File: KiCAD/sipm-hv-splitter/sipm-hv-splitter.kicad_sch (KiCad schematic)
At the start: 16 parts, among them J1 Conn_02x18_Odd_Even, J2 Conn_02x17_Odd_Even, J3 -OMIT-, U1 ATmega328-M, U14 TPS7A25, U16 TPS7A25

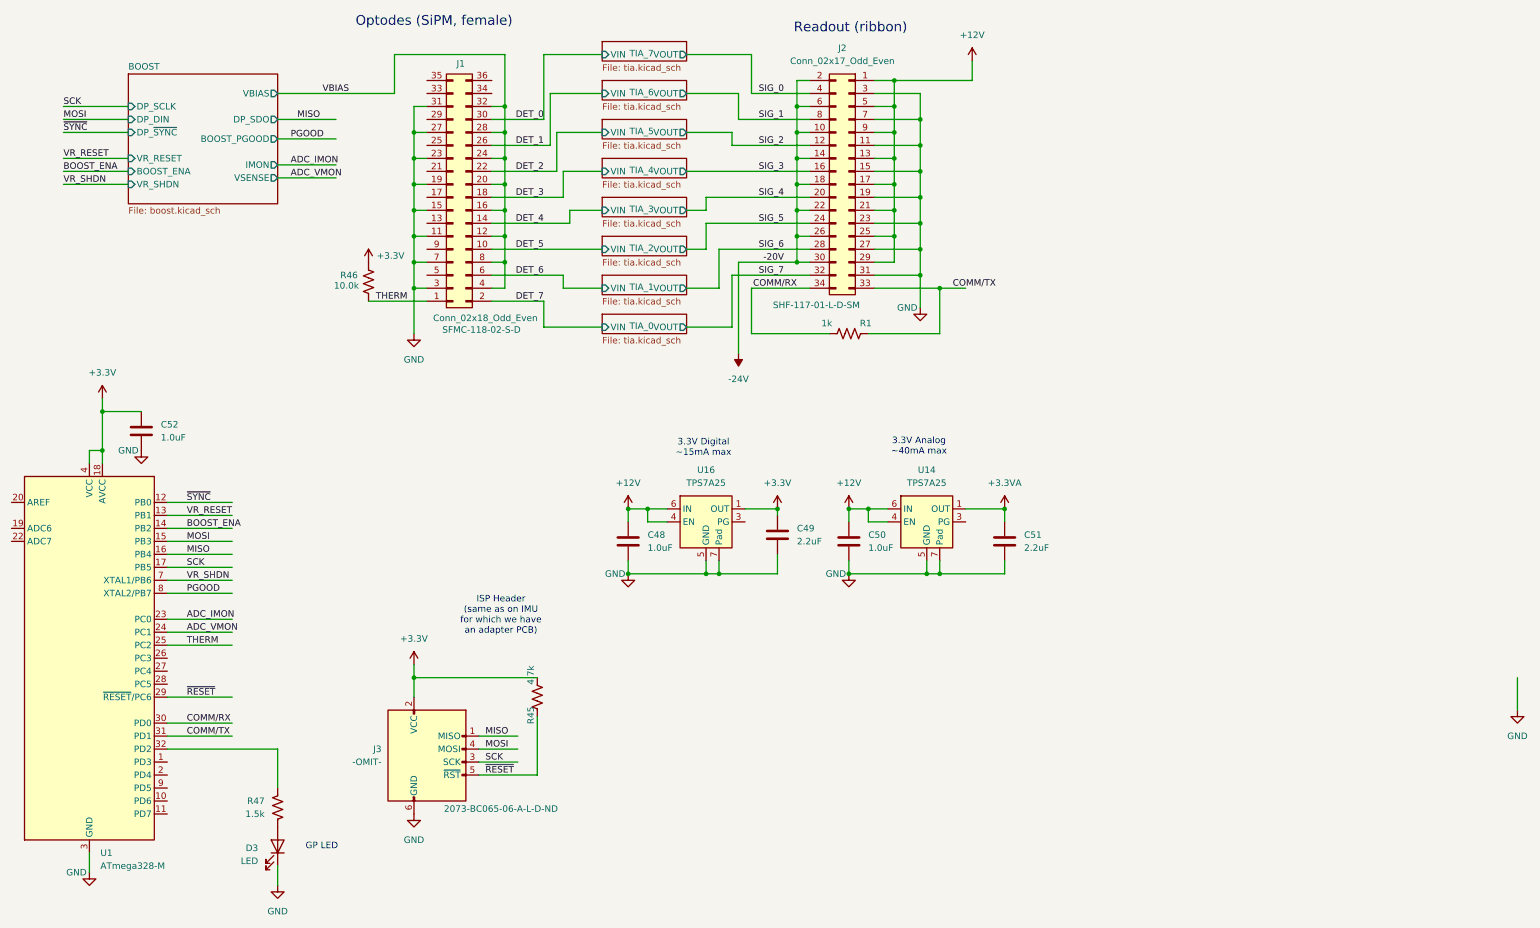
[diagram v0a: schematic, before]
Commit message: working on bias filter changes
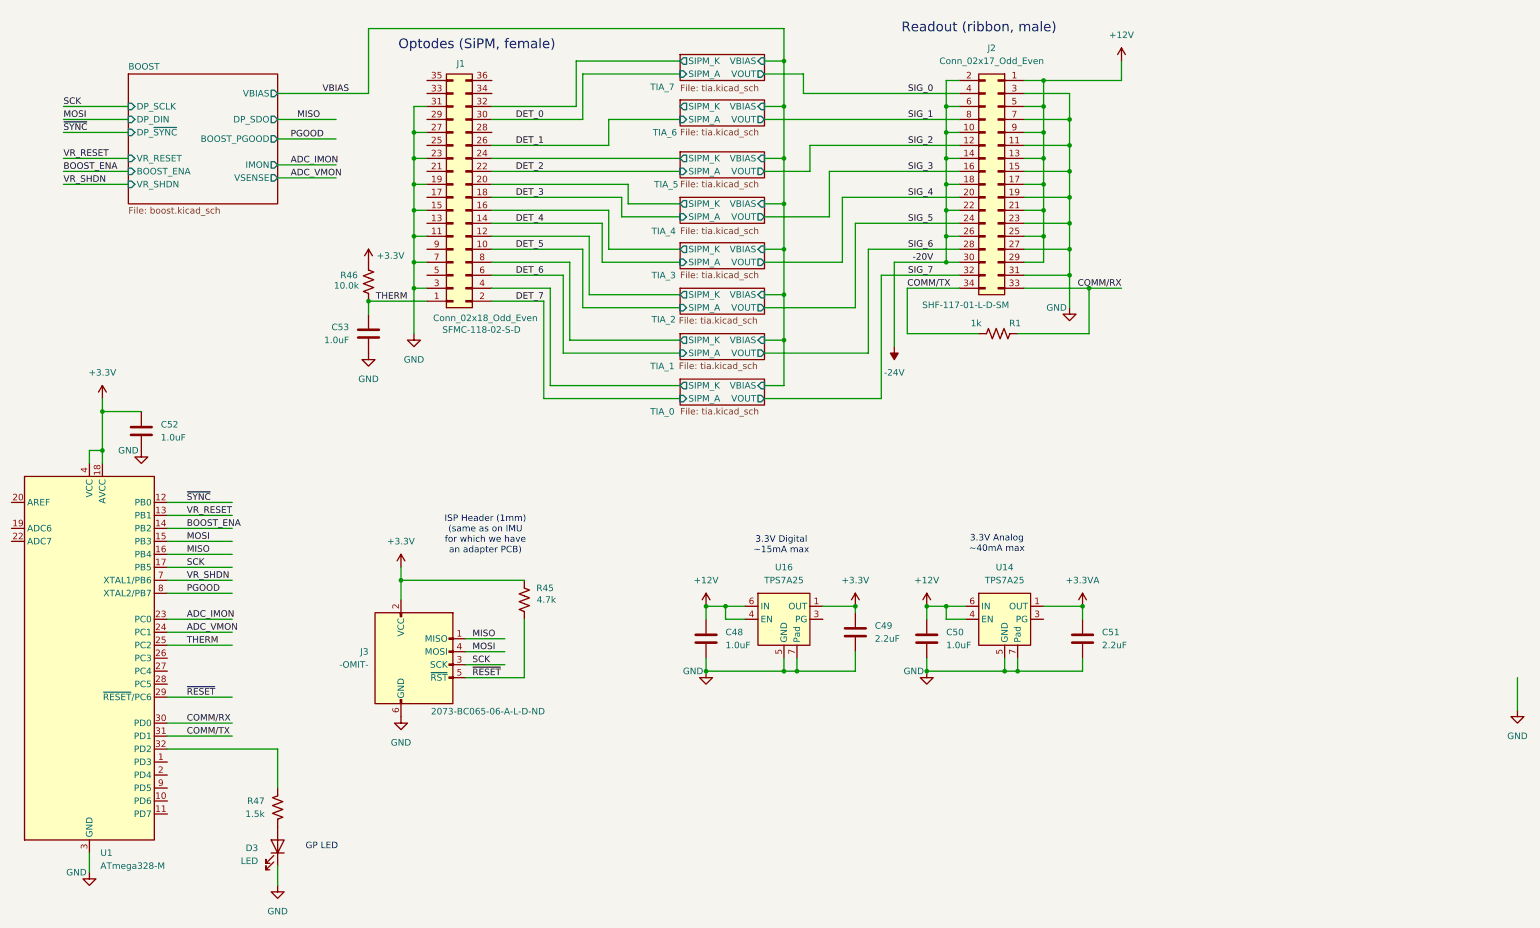
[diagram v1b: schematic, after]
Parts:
- added C53: 1.0uF, Capacitor_SMD:C_0603_1608Metric_Pad1.08x0.95mm_HandSolder, symbol Device:C
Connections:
- net COMM/RX: now also J2.33 (Pin_33), R1.1; no longer J2.34 (Pin_34), R1.2
- net COMM/TX: now also J2.34 (Pin_34), R1.2; no longer J2.33 (Pin_33), R1.1
- net GND: now also C53.2
- net THERM: now also C53.1
- net VBIAS: no longer J1.12 (Pin_12), J1.16 (Pin_16), J1.20 (Pin_20), J1.24 (Pin_24), J1.28 (Pin_28), J1.32 (Pin_32), J1.4 (Pin_4), J1.8 (Pin_8)
- new net TIA_0/SIPM_K: J1.4 (Pin_4)
- new net TIA_1/SIPM_K: J1.8 (Pin_8)
- new net TIA_2/SIPM_K: J1.12 (Pin_12)
- new net TIA_3/SIPM_K: J1.16 (Pin_16)
- new net TIA_4/SIPM_K: J1.20 (Pin_20)
- new net TIA_5/SIPM_K: J1.24 (Pin_24)
- new net TIA_7/SIPM_K: J1.32 (Pin_32)
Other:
- sheet TIA_0 ports: added SIPM_A, SIPM_K, VBIAS; removed VIN
- sheet TIA_1 ports: added SIPM_A, SIPM_K, VBIAS; removed VIN
- sheet TIA_2 ports: added SIPM_A, SIPM_K, VBIAS; removed VIN
- sheet TIA_3 ports: added SIPM_A, SIPM_K, VBIAS; removed VIN
- sheet TIA_4 ports: added SIPM_A, SIPM_K, VBIAS; removed VIN
- sheet TIA_5 ports: added SIPM_A, SIPM_K, VBIAS; removed VIN
- sheet TIA_6 ports: added SIPM_A, SIPM_K, VBIAS; removed VIN
- sheet TIA_7 ports: added SIPM_A, SIPM_K, VBIAS; removed VIN
- note added: "ISP Header (1mm) (same as on IMU for which we have an adapter PCB)"
- note added: "Readout (ribbon, male)"
- note removed: "ISP Header (same as on IMU for which we have an adapter PCB)"
- note removed: "Readout (ribbon)"
- moved on the sheet: C48, C49, C50, C51, J2, J3, R1, R45, U14, U16
